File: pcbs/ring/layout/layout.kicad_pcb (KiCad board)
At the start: 2 copper layers, 57 x 6.2 mm, 65 parts, among them J1 ?, Q1 CSD13380F3T, Q2 CSD13380F3T, U1 BQ27427YZFR, U2 BQ29700, U3 nRF52833-QDAA, U4 MAX30102EFD+T, U5 LSM6DSOX, U6 TMP117AIDRVR, U7 TPS7A2018PDQN, Y1 32MHz, Y2 32.768kHz

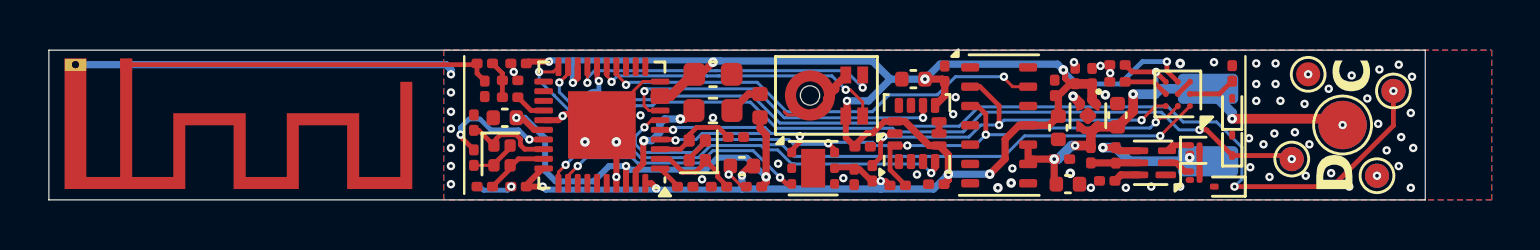
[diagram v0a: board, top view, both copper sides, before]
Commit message: cleanup
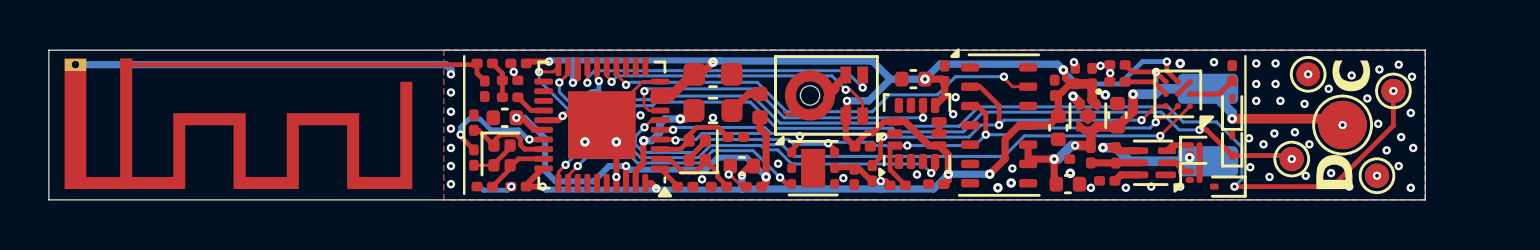
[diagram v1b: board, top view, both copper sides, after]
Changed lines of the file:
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@@
 		(net 2)
 		(net_name "GND")
-		(locked yes)
 		(layers "F.Cu" "B.Cu")
 		(hatch edge 0.5)
@@
 		(polygon
 			(pts
-				(xy 134.6 80) (xy 178 80) (xy 178 86.2) (xy 134.6 86.2)
+				(xy 134.6 80) (xy 175.25 80) (xy 175.25 86.2) (xy 134.6 86.2)
 			)
 		)
